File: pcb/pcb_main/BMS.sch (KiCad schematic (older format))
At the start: 26 parts, among them Q1 PZT3906, SW2 SW_SPDT, U4 MCP73833, U5 LM8364-2.2, U6 LTC3525-5

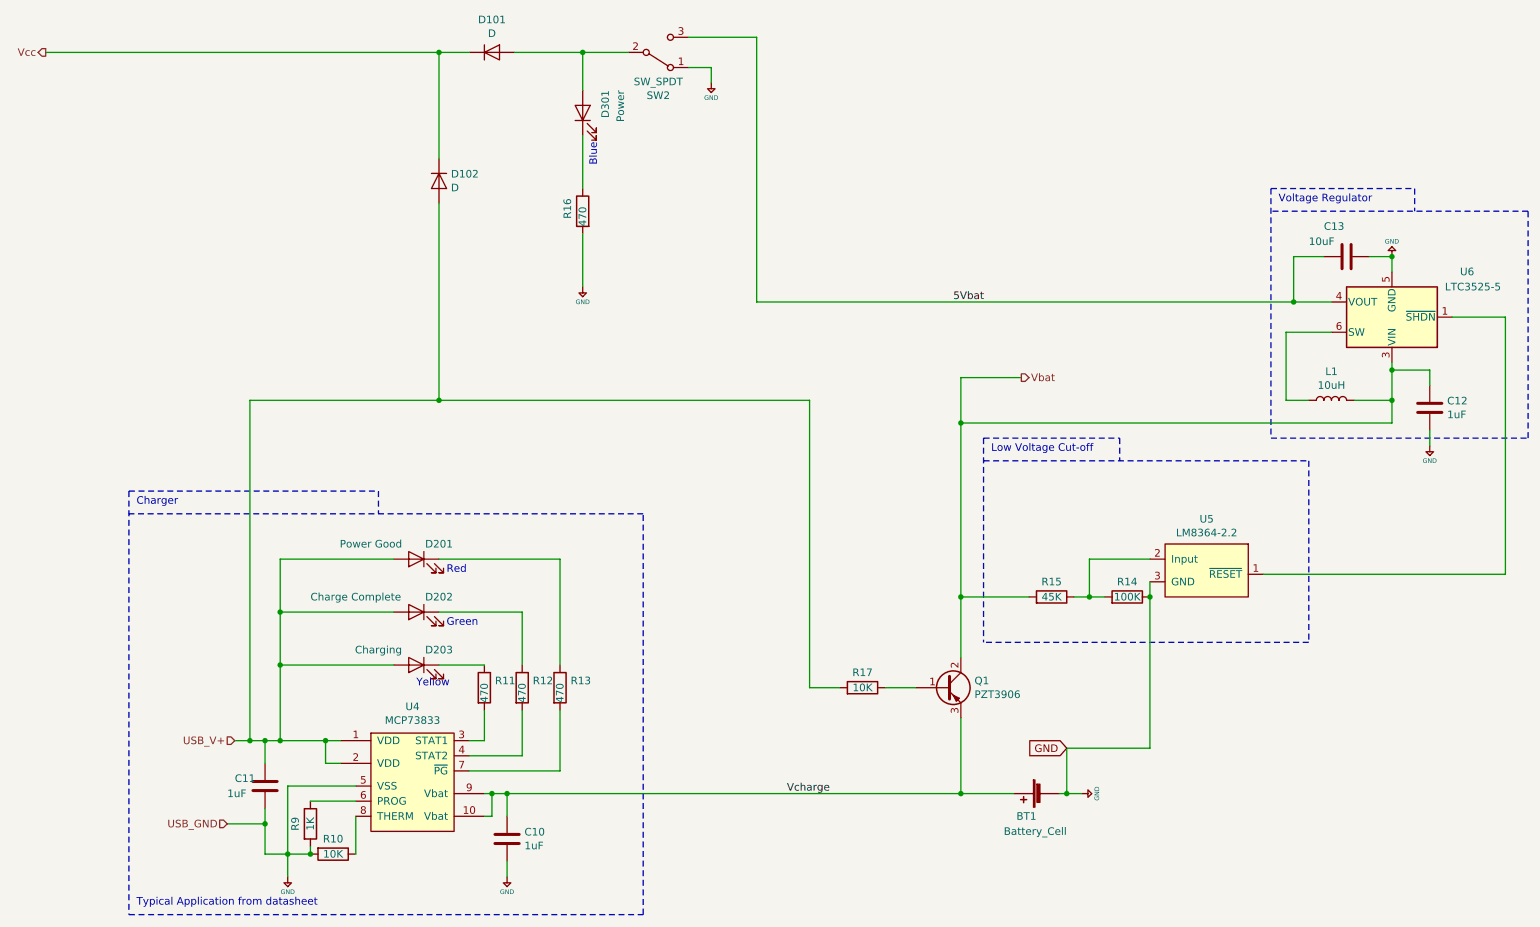
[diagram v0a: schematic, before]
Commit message: bms changes
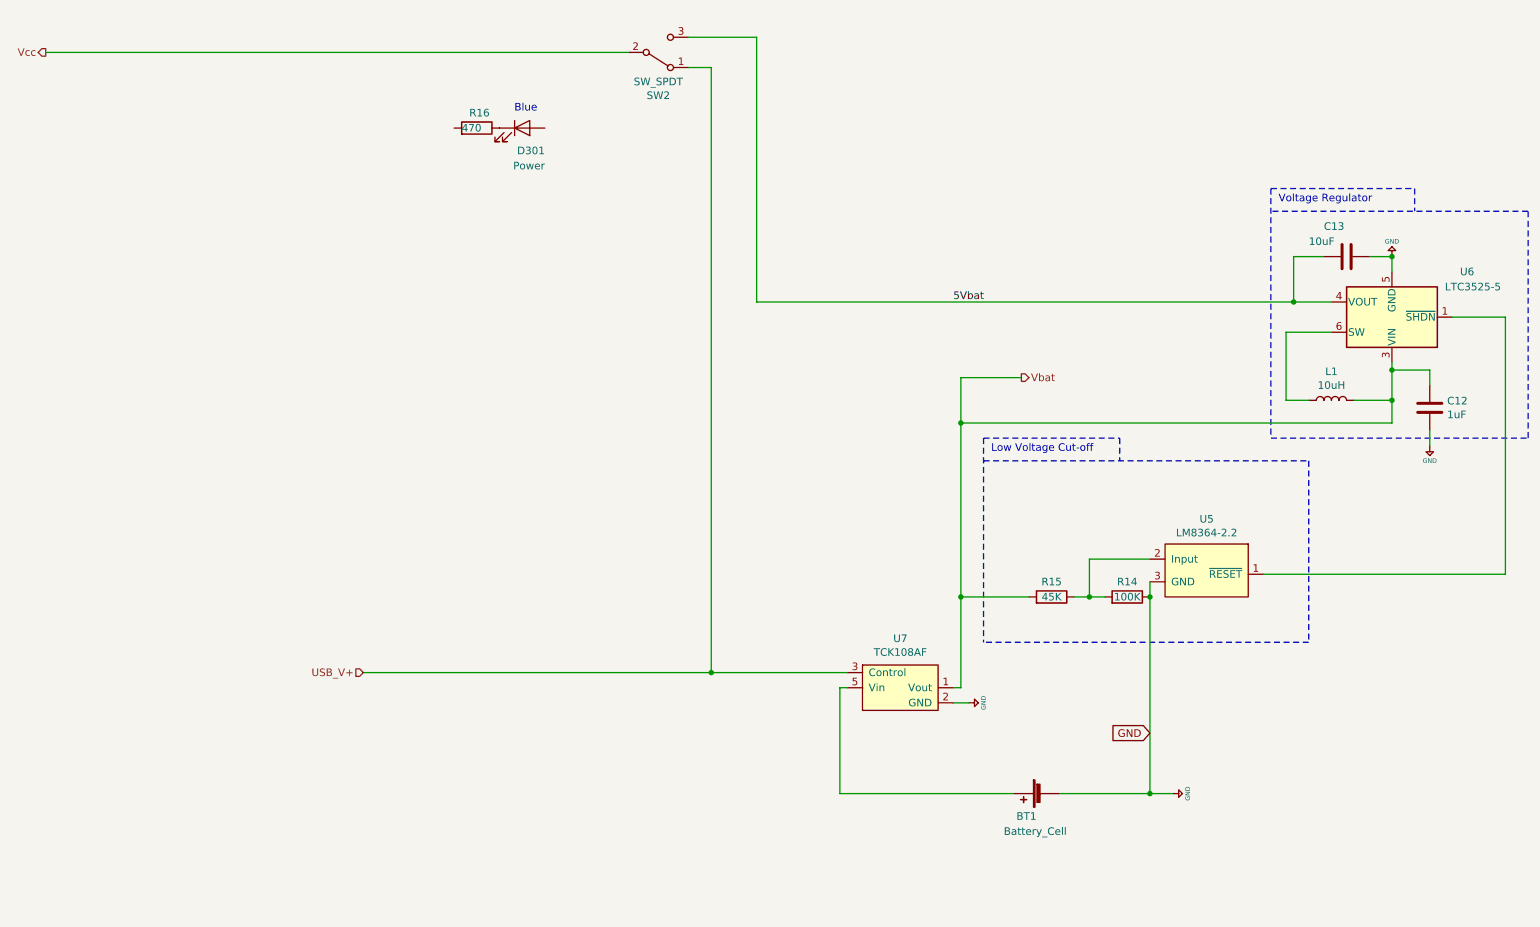
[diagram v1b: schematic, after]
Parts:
- removed C10, C11: 1uF, Capacitor_SMD:C_0805_2012Metric_Pad1.15x1.40mm_HandSolder, symbol Device:C
- removed D101, D102: D, SVastaCustomParts:D_MiniMELF_Handsoldering_Shorter_Pads, symbol Device:D
- removed D201: Power Good, LED_SMD:LED_0805_2012Metric_Pad1.15x1.40mm_HandSolder, symbol Device:LED
- removed D202: Charge Complete, LED_SMD:LED_0805_2012Metric_Pad1.15x1.40mm_HandSolder, symbol Device:LED
- removed D203: Charging, LED_SMD:LED_0805_2012Metric_Pad1.15x1.40mm_HandSolder, symbol Device:LED
- removed Q1: PZT3906, Package_TO_SOT_SMD:SOT-223, symbol Transistor_BJT:PZT3906
- removed R10, R17: 10K, Resistor_SMD:R_0805_2012Metric_Pad1.15x1.40mm_HandSolder, symbol Device:R
- removed R11, R12, R13: 470, Resistor_SMD:R_0805_2012Metric_Pad1.15x1.40mm_HandSolder, symbol Device:R
- removed R9: 1K, Resistor_SMD:R_0805_2012Metric_Pad1.15x1.40mm_HandSolder, symbol Device:R
- removed U4: MCP73833, SVastaCustomParts:MCP73833T-AMI-UN, symbol SVastaCustomParts:MCP73833
- added U7: TCK108AF, symbol SVastaCustomParts:TCK108AF
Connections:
- net +5V: now also U7.2 (GND); no longer R16.2, SW2.1 (A)
- net USB_V+: now also SW2.1 (A), U7.3 (Control)
- net Vbat: now also U7.1 (Vout)
- net Vcc: now also SW2.2 (B)
- net at D301.2 (A): no longer SW2.2 (B)
- net Vcharge: no longer names the net of BT1.1 (+)
- net Vcharge: now also U7.5 (Vin)
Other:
- note removed: "Charger"
- note removed: "Green"
- note removed: "Red"
- note removed: "Typical Application from datasheet"
- note removed: "Yellow"
- moved on the sheet: D301, R16
